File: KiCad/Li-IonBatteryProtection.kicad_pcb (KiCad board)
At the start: 2 copper layers, 179.1 x 54.6 mm, 55 parts, among them J1 CONN_02X03, J2 CONN_01X02, Q1 IRF540N, Q2 2N2222A, Q3 2N2222A, Q4 2N2222A, Q5 2N2222A, Q6 2N2222A, U1 LM311N, U2 PC817, U3 LM311N, U4 PC817, U5 LM311N, U6 PC817, U7 LM311N, U8 PC817

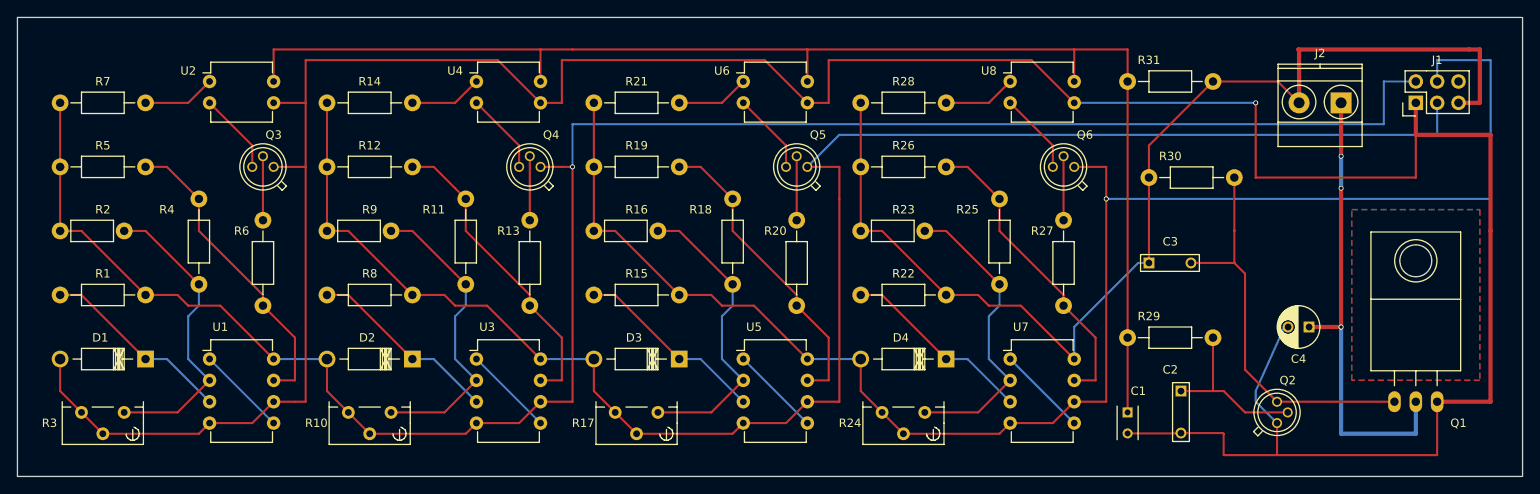
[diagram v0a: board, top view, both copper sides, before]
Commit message: Hopefully finished the PCB.
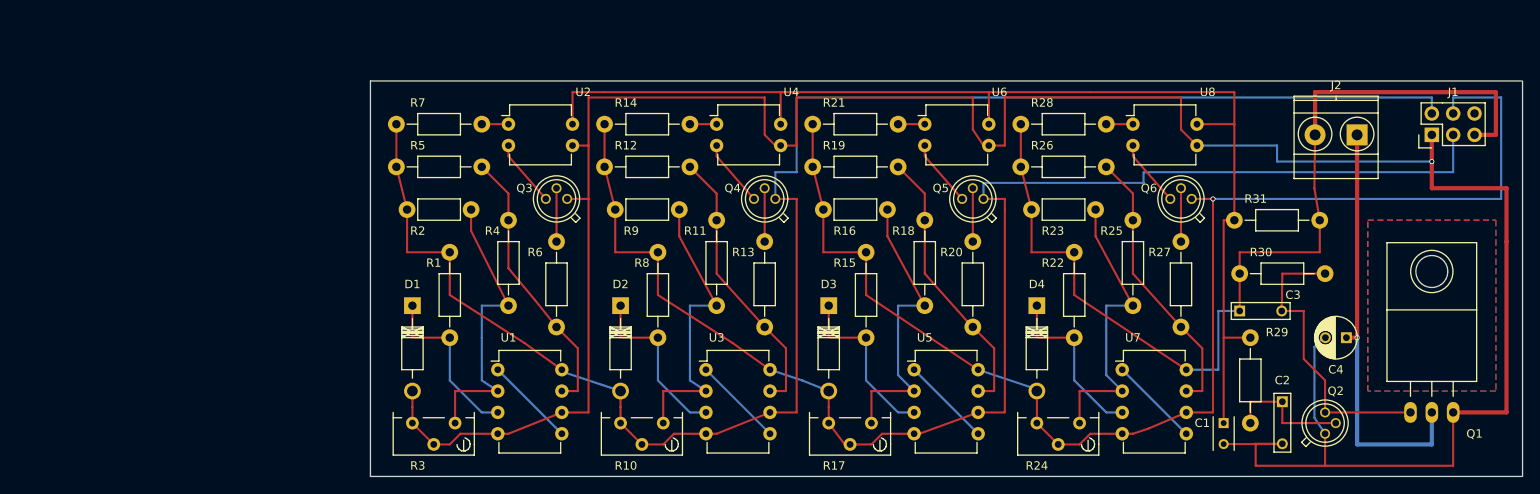
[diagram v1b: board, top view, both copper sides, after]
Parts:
- moved R2 41.4 mm to (98.4, 95.2)
- moved R7 40.1 mm to (97.2, 85.1)
- moved R5 40.0 mm to (97.2, 90.2)
- moved R3 39.4 mm to (104.1, 120.7)
- moved R4 36.9 mm to (110.5, 96.5)
- moved R1 36.5 mm to (103.5, 100.3), turned to 270 degrees
- moved U2 35.9 mm to (110.5, 85.1)
- moved Q3 35.1 mm to (116.2, 94.0)
- moved R6 35.0 mm to (116.2, 99.1)
- moved R9 34.4 mm to (123.2, 95.2)
- moved U1 34.3 mm to (109.2, 114.3)
- moved R14 33.1 mm to (121.9, 85.1)
- moved R12 33.0 mm to (121.9, 90.2)
- moved R10 32.4 mm to (128.9, 120.7)
- moved D1 32.4 mm to (99.1, 106.7), turned to 270 degrees
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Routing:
- net Battery-GND: track 361.4 -> 304.7 mm
- net Battery-1: track 232.2 -> 196.5 mm, vias 1 -> 0
- net Battery-2: track 202.1 -> 167.5 mm
- net Battery-3: track 192.9 -> 158.4 mm
- net Net-(C1-Pad1): track 160.0 -> 138.4 mm
- net Battery-4: track 135.7 -> 120.9 mm
- net Net-(C3-Pad2): track 48.0 -> 35.4 mm
- net Net-(R14-Pad2): track 8.67 -> 3.17 mm
- net Net-(R28-Pad2): track 8.67 -> 3.17 mm
- net Net-(R7-Pad2): track 8.67 -> 3.17 mm
- net Net-(R21-Pad2): track 8.67 -> 3.18 mm
- net Net-(C4-Pad1): track 55.9 -> 50.8 mm, vias 3 -> 1
- net Net-(C2-Pad1): track 20.1 -> 15.2 mm
- net Net-(R4-Pad1): track 36.8 -> 33.0 mm
- net Net-(R11-Pad1): track 36.8 -> 33.1 mm
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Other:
- board size 179.1 x 54.6 mm -> 137.1 x 47 mm
